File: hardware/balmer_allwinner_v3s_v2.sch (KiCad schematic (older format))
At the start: 32 parts, among them U1 AllwinnerV3S

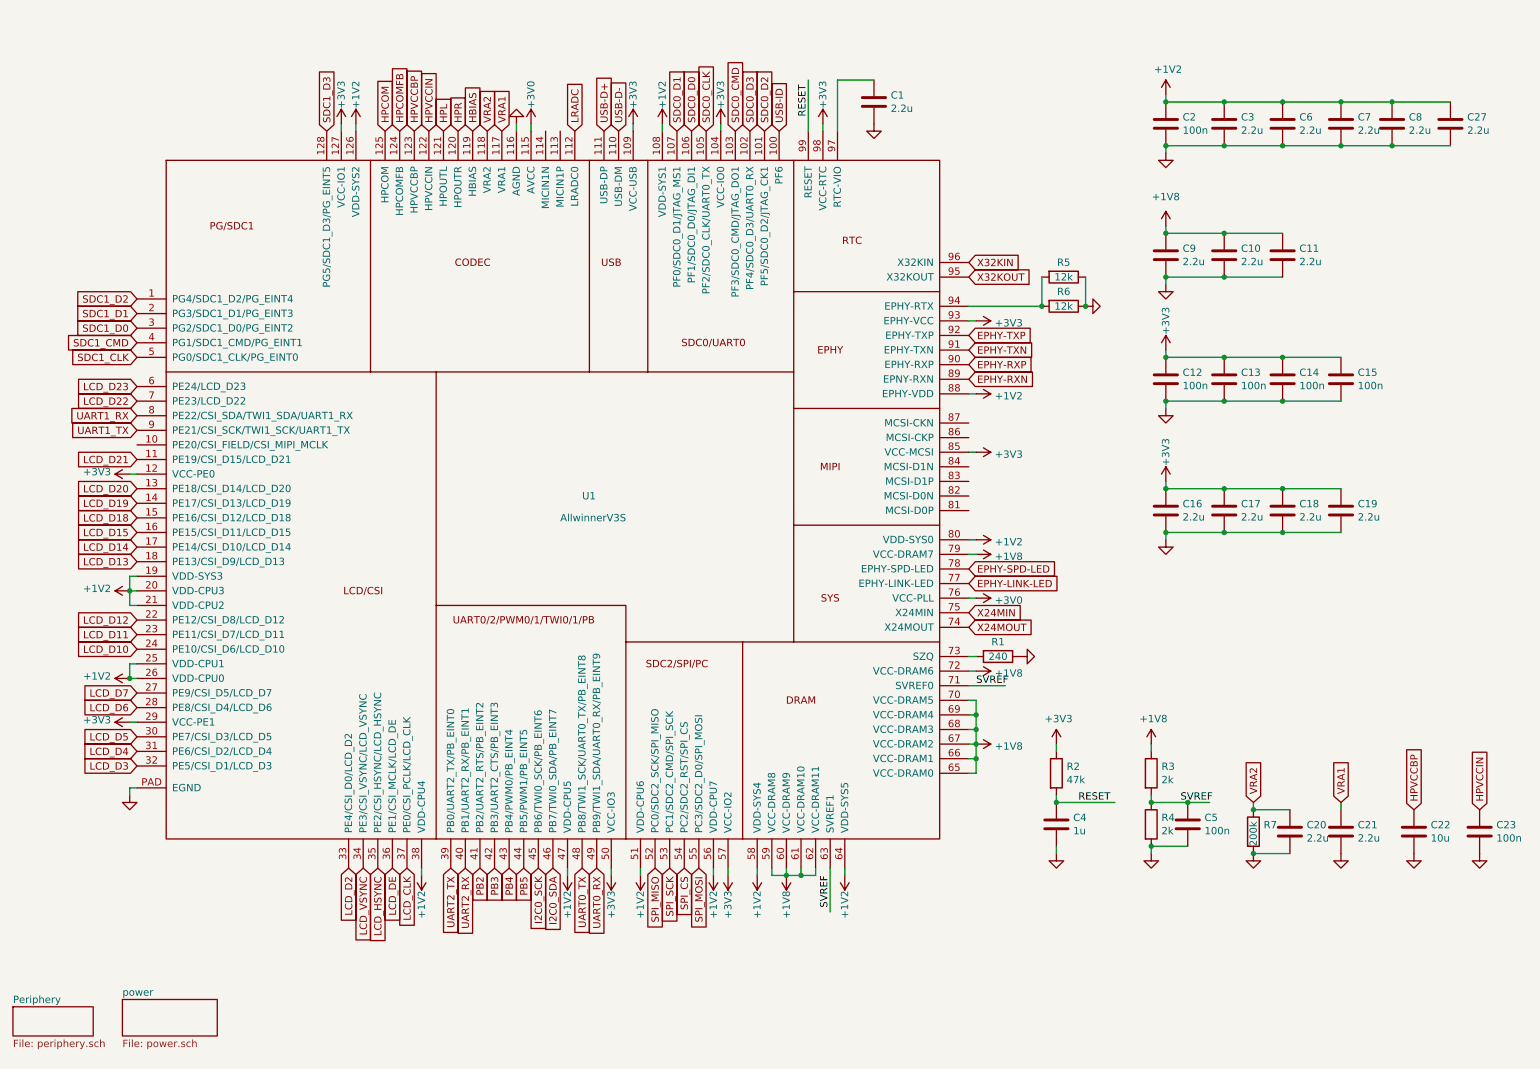
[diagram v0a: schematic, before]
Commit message: Some routing done
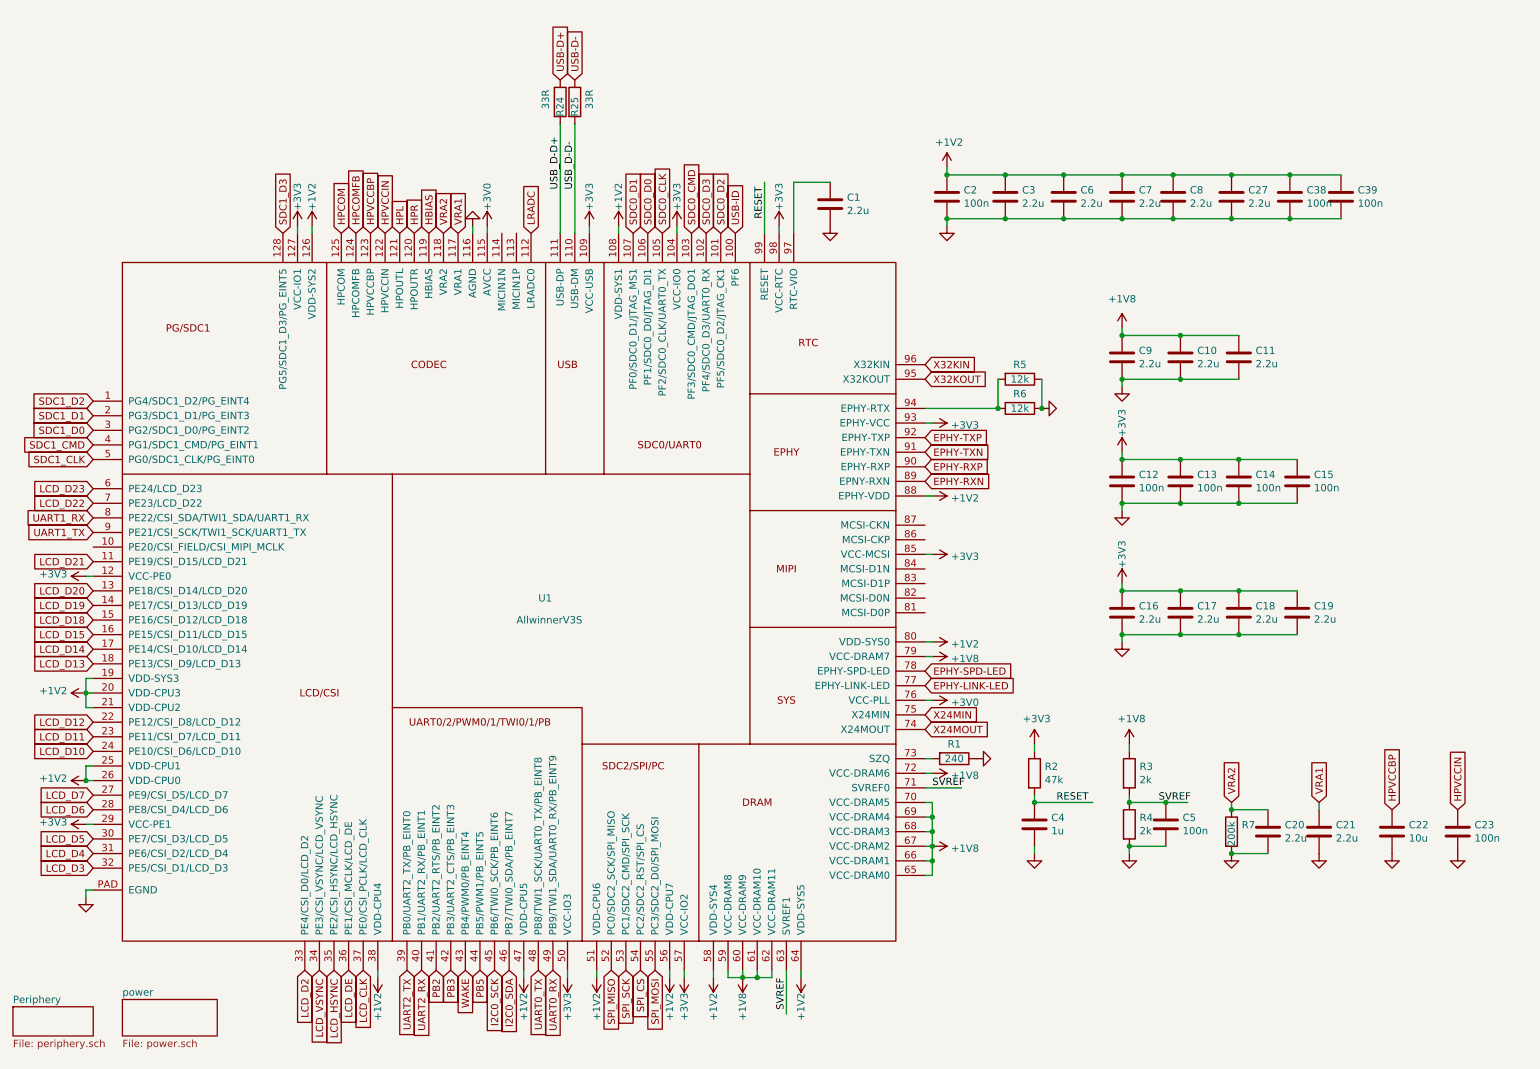
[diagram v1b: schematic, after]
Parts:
- added C38, C39: 100n, Capacitor_SMD:C_0603_1608Metric, symbol Device:C
- added R24, R25: 33R, Resistor_SMD:R_0603_1608Metric, symbol Device:R
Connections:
- net labels added: USB_D-D+, USB_D-D-, WAKE
- net labels removed: PB4
- wire segments 110 -> 116
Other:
- moved on the sheet: C1, C10, C11, C12, C13, C14, C15, C16, C17, C18, C19, C2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
